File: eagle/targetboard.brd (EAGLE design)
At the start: 99.7 x 49.5 mm, 74 parts, among them CN1 DIP-BLACK-MALE-HEADER-VERT(3P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, IC1 TB6612FNG, IC2 TB6612FNG, IC3 MCP2551, IC4 MCP2551, IC5 LPC1768 or LPC1768, IC6 PMIC-CJT1117-3.3(SOT223), IC7 MAX232D, J1 USB, J2 Serial, J3 CAN, J4 2x8p-2.54, J5 2x8p-2.54, J6 DIP-BLACK-MALE-HEADER-VERT(8P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, J7 2x8p-2.54, Q1 PNP-24V, SW1 SW, Y1 12MHZ

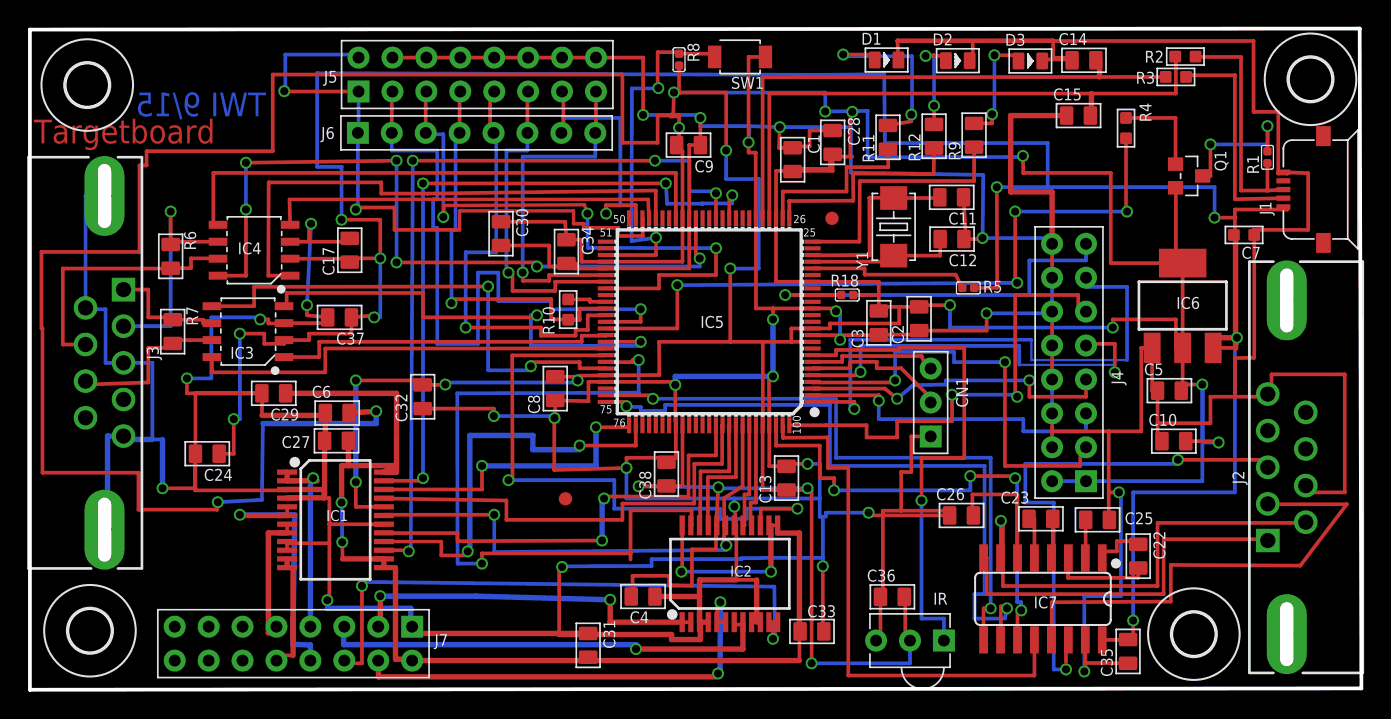
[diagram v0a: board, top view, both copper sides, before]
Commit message: Update of board
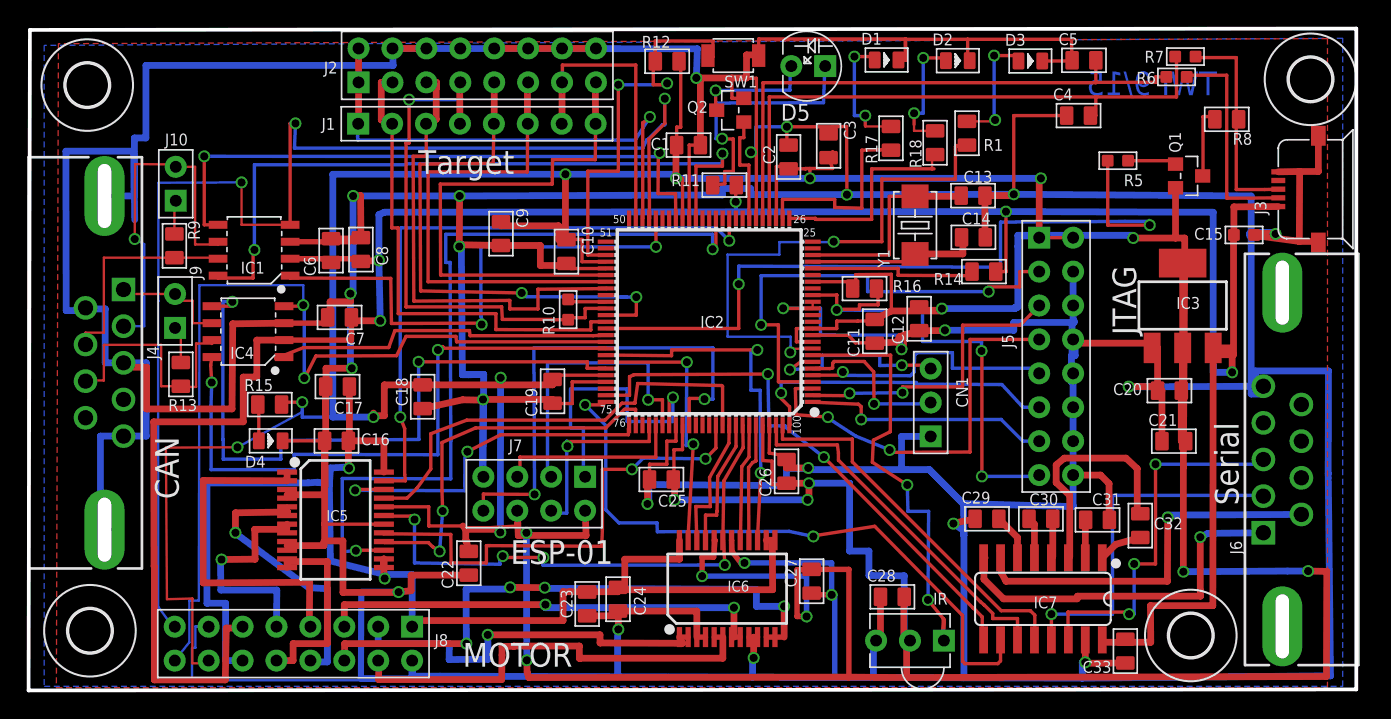
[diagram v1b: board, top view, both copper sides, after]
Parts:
- removed C34, C35, C37, C38: 100nf, Seeed-OPL-Capacitor:C0805
- removed C36: 10uf, Seeed-OPL-Capacitor:C0805
- removed R2, R3: 33.2R, Seeed-OPL-Resistor:R0603
- removed R4: 51R, Seeed-OPL-Resistor:R0603
- removed U$4, U$5: (no value), dicons:FIDUCIAL_G10
- added C16, C18, C21: 10uf, Seeed-OPL-Capacitor:C0805
- added C19, C20: 100nf, Seeed-OPL-Capacitor:C0805
- added D4: SMD-LED-CLEAR-RED(0805), Seeed-OPL-Diode:LED-0805
- added D5: IR 940NM, Seeed-OPL-Diode:LED2-2.54-D5.0MM
- added J10: CAN1, Seeed-OPL-Connector:H2-2.54
- added J8: 2x8p-2.54, Seeed-OPL-Connector:H2X8-2.54
- added J9: CAN2, Seeed-OPL-Connector:H2-2.54
- added Q2: NMOSFET, Seeed-OPL-Transistor:SOT-23
- added R13: 120R, Seeed-OPL-Resistor:R0805
- added R14: 1.5K, Seeed-OPL-Resistor:R0805
- added R15: 100R, Seeed-OPL-Resistor:R0805
- added R16: 2K, Seeed-OPL-Resistor:R0805
- added R17: 390R, Seeed-OPL-Resistor:R0805
- C10, C27: value 10uf -> 100nf
- C11, C12: value 18pf -> 100nf
- C13, C4, C5: value 100nf -> 18pf
- C15: value 18pf -> 10uf; device Seeed-OPL-Capacitor:C0805 -> Seeed-OPL-Capacitor:C0603
- C22, C23, C25, C26: value 1uf -> 100nf
- C24: value 1uf -> 10uf
- C29, C30, C6: value 100nf -> 1uf
- C3: value 100nf -> 10uf
- C31, C32: value 10uf -> 1uf
- C7: value 10uf -> 100nf; device Seeed-OPL-Capacitor:C0603 -> Seeed-OPL-Capacitor:C0805
- IC1: value TB6612FNG -> MCP2551; device Seeed-OPL-ic:SSOP24-0.65-8.9X5.3MM -> Seeed-OPL-ic:SOIC8-1.27-5X4MM
- IC2: value TB6612FNG -> LPC1768 or LPC1768; device Seeed-OPL-ic:SSOP24-0.65-8.9X5.3MM -> Seeed-OPL-ic:LQFP100-0.5-13.8X13.8MM
- IC3: value MCP2551 -> PMIC-CJT1117-3.3(SOT223); device Seeed-OPL-ic:SOIC8-1.27-5X4MM -> Seeed-OPL-ic:SOT-223
- IC5: value LPC1768 or LPC1768 -> TB6612FNG; device Seeed-OPL-ic:LQFP100-0.5-13.8X13.8MM -> Seeed-OPL-ic:SSOP24-0.65-8.9X5.3MM
- IC6: value PMIC-CJT1117-3.3(SOT223) -> TB6612FNG; device Seeed-OPL-ic:SOT-223 -> Seeed-OPL-ic:SSOP24-0.65-8.9X5.3MM
- J1: value USB -> DIP-BLACK-MALE-HEADER-VERT(8P-2.54); device Seeed-OPL-Connector:MICRO-USB5+2P-SMD-0.65 -> Seeed-OPL-Connector:H8-2.54
- J2: value Serial -> 2x8p-2.54; device Seeed-OPL-Connector:DSUB9+2P-2.77-90D-MALE -> Seeed-OPL-Connector:H2X8-2.54
- J3: value CAN -> USB; device Seeed-OPL-Connector:DSUB9+2P-2.77-90D-MALE -> Seeed-OPL-Connector:MICRO-USB5+2P-SMD-0.65
- J4: value 2x8p-2.54 -> CAN; device Seeed-OPL-Connector:H2X8-2.54 -> Seeed-OPL-Connector:DSUB9+2P-2.77-90D-MALE
- J6: value DIP-BLACK-MALE-HEADER-VERT(8P-2.54) -> Serial; device Seeed-OPL-Connector:H8-2.54 -> Seeed-OPL-Connector:DSUB9+2P-2.77-90D-MALE
- J7: value 2x8p-2.54 -> 2X4P-2.54; device Seeed-OPL-Connector:H2X8-2.54 -> Seeed-OPL-Connector:H2X4-2.54
- R1, R18: value 1.5K -> 390R; device Seeed-OPL-Resistor:R0402 -> Seeed-OPL-Resistor:R0805
- R11: value 2K -> 100R
- R12: value 2K -> 1.5K
- R5: value 1.5K -> 51R; device Seeed-OPL-Resistor:R0402 -> Seeed-OPL-Resistor:R0603
- R6, R7: value 120R -> 33.2R; device Seeed-OPL-Resistor:R0805 -> Seeed-OPL-Resistor:R0603
- R8: device Seeed-OPL-Resistor:R0402 -> Seeed-OPL-Resistor:R0805
- R9: value 2K -> 120R
- moved H3 100.3 mm to (4.78, 4.42)
- moved H4 92.4 mm to (87.2, 4.06)
- moved J3 88.9 mm to (93.8, 37.5), turned to 90 degrees
- moved R7 78.6 mm to (86.8, 47.4), turned to 90 degrees
- moved R6 76.5 mm to (86.2, 45.9), turned to 90 degrees
- moved J4 72.2 mm to (5.87, 24.5), turned to 270 degrees
- moved IC3 70.0 mm to (86.6, 28.8), turned to 0 degrees
- moved C7 68.0 mm to (23.5, 27.9)
- moved J2 67.7 mm to (33.8, 46.8)
- moved J6 65.1 mm to (94.1, 17.2)
- moved J1 60.6 mm to (33.8, 42.4)
- moved R9 60.5 mm to (11.1, 33.2), turned to 0 degrees
- moved C32 54.6 mm to (83.4, 12.3)
- moved C29 54.2 mm to (72.0, 12.8), turned to 90 degrees
- moved C22 50.1 mm to (33.1, 9.47), turned to 180 degrees
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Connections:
- removed net N$12: IC5.98, IC7.11
- removed net N$28: J7.11
- removed net N$29: J7.10
- removed net N$30: J7.9
- removed net N$31: J7.8
- removed net N$32: J7.7
- removed net N$33: J7.6
- new net ESP_0: IC2.81, J7.2
- new net ESP_2: IC2.80, J7.3
- new net ESP_RST: IC2.79, J7.7
- new net IR_SEND: IC2.32, Q2.1
- new net N$11: J10.1, R9.1
- new net N$14: D5.+, R11.1
- new net N$21: D5.-, Q2.3
- new net N$24: D4.+, R15.1
- new net RXD0: IC2.99, IC7.12
- new net RX_TO_TX: IC2.85, J7.5
- new net TXD0: IC2.98, IC7.11
- new net TX_TO_RX: IC2.82, J7.1
- net +12V: now also C16.2, C17.1, C23.1, C24.2, IC5.13, IC5.14, IC5.24, IC6.13, IC6.14, IC6.24, J8.1, J8.11; no longer C27.2, C29.1, C31.2, C33.1, IC1.13, IC1.14, IC1.24, IC2.13, IC2.14, IC2.24, J7.16
- net CAN1_H: now also IC1.7, J4.7, R9.2; no longer IC4.7, J3.7, R6.2
- net CAN1_L: now also IC1.6, J10.2, J4.2; no longer IC4.6, J3.2, R6.1
- net CAN1_REF: now also IC1.5, IC2.43; no longer IC4.5, IC5.43
- net CAN1_RS: now also IC1.8, IC2.40; no longer IC4.8, IC5.40
- net CAN1_RX: now also IC1.4, IC2.47, J8.8; no longer IC4.4, IC5.47
- net CAN1_TX: now also IC1.1, IC2.46; no longer IC4.1, IC5.46
- net CAN2_H: now also IC4.7, J4.8, R13.2; no longer IC3.7, J3.8, R7.2
- net CAN2_L: now also IC4.6, J4.1, J9.2; no longer IC3.6, J3.1, R7.1
- net CAN2_REF: now also IC2.70, IC4.5; no longer IC3.5, IC5.70
- net CAN2_RS: now also IC2.67, IC4.8; no longer IC3.8, IC5.67
- net CAN2_RX: now also IC2.66, IC4.4, J8.9; no longer IC3.4, IC5.66
- net CAN2_TX: now also IC2.65, IC4.1; no longer IC3.1, IC5.65
- net CM1A: now also IC2.91, IC6.22; no longer IC2.22, IC5.91
- net CM1B: now also IC2.92, IC6.21; no longer IC2.21, IC5.92
- net CM2A: now also IC2.94, IC6.17; no longer IC2.17, IC5.94
- net CM2B: now also IC2.95, IC6.16; no longer IC2.16, IC5.95
- net CM3A: now also IC2.76, IC5.22; no longer IC1.22, IC5.76
- net CM3B: now also IC2.90, IC5.21; no longer IC1.21, IC5.90
- net CM4A: now also IC2.89, IC5.17; no longer IC1.17, IC5.89
- net CM4B: now also IC2.77, IC5.16; no longer IC1.16, IC5.77
- net DM: now also J3.2, R6.2; no longer J1.2, R3.2
- net DP: now also J3.3, R7.2, R8.1; no longer J1.3, R1.1, R2.2
- net EDM: now also C5.2, IC2.30, R6.1; no longer C14.2, IC5.30, R3.1
- net EDP: now also C4.2, IC2.29, R7.1; no longer C15.2, IC5.29, R2.1
- net GND: now also C10.2, C13.1, C16.1, C18.1, C19.1, C20.1, C21.1, C22.1, C23.2, C24.1, C26.2, C29.1, C31.2, C33.1, C6.2, C7.2, C8.2, C9.2, D4.-, IC2.11, IC2.15, IC2.16, IC2.31, IC2.41, IC2.55, IC2.72, IC2.83, IC2.97, IC3.1, IC5.10, IC5.18, IC5.3, IC5.4, IC5.9, IC6.10, IC6.18, IC6.3, IC6.4, IC6.9, J2.10, J2.11, J2.12, J2.13, J2.14, J2.15, J2.9, J3.7, J4.3, J4.5, J4.6, J4.G1, J4.G2, J6.5, J7.4, J8.16, J8.7, Q2.2; no longer C10.1, C13.2, C24.2, C26.1, C29.2, C30.2, C31.1, C32.1, C33.2, C34.2, C35.1, C36.1, C37.2, C38.2, C6.1, C7.1, C8.1, C9.1, IC1.10, IC1.18, IC1.4, IC1.9, IC2.10, IC2.18, IC2.3, IC2.4, IC2.9, IC3.3, IC5.11, IC5.15, IC5.31, IC5.41, IC5.55, IC5.72, IC5.83, IC5.97, IC6.1, J1.5, J2.5, J2.7, J3.3, J3.G1, J3.G2, J4.10, J4.11, J4.12, J4.13, J4.14, J4.15, J4.9, J7.1
- net IR_IN: now also IC2.8; no longer IC5.8
- net LED1: now also IC2.9, R1.1; no longer IC5.25, R9.1
- net LED2: now also IC2.27, R17.1; no longer IC5.27, R11.1
- net LED3: now also IC2.26, R18.1; no longer IC5.26, R12.1
- net M1A: now also IC6.1, IC6.2, J8.2; no longer IC2.1, IC2.2, J7.2
- net M1B: now also IC6.5, IC6.6, J8.15; no longer IC2.5, IC2.6, J7.15
- net M2A: now also IC6.7, IC6.8, J8.3; no longer IC2.7, IC2.8, J7.3
- net M2B: now also IC6.11, IC6.12, J8.14; no longer IC2.11, IC2.12, J7.14
- net M3A: now also IC5.1, IC5.2, J8.4; no longer IC1.1, IC1.2, J7.4
- net M3B: now also IC5.5, IC5.6, J8.13; no longer IC1.5, IC1.6, J7.13
- net M4A: now also IC5.7, IC5.8, J8.5; no longer IC1.7, IC1.8, J7.5
- net M4B: now also IC5.11, IC5.12, J8.12; no longer IC1.11, IC1.12, J7.12
- net N$1: now also IC2.48, J1.1, J2.1, J2.16; no longer IC5.48, J5.1, J5.16, J6.1
- net N$10: now also IC2.21, R14.2; no longer IC5.21, R5.1
- net N$13: now also J9.1, R13.1; no longer IC5.99, IC7.12
- net N$15: now also C30.2; no longer C23.2
- net N$16: now also C30.1; no longer C23.1
- net N$17: now also C32.1; no longer C22.1
- net N$18: now also C32.2; no longer C22.2
- net N$19: now also C29.2; no longer C26.2
- net N$2: now also IC2.53, R12.1; no longer IC5.53, R8.1
- net N$20: now also C31.1; no longer C25.1
- net N$22: now also IC2.60; no longer IC5.60
- net N$3: now also R18.2; no longer R12.2
- net N$4: now also R17.2; no longer R11.2
- net N$5: now also R1.2; no longer R9.2
- net N$6: now also C14.2, IC2.22; no longer C12.2, IC5.22
- net N$7: now also R8.2; no longer R1.2
- net N$8: now also C13.2, IC2.23; no longer C11.2, IC5.23
- net N$9: now also R5.2; no longer R4.2
- net NTRST: now also IC2.4, J5.2; no longer IC5.4, J4.2
- net P2_9: now also IC2.64, R5.1; no longer IC5.64, R4.1
- net PWM1: now also IC2.69, IC6.23; no longer IC2.23, IC5.69
- net PWM2: now also IC2.68, IC6.15; no longer IC2.15, IC5.68
- net PWM3: now also IC2.35, IC5.23; no longer IC1.23, IC5.35
- net PWM4: now also IC2.37, IC5.15; no longer IC1.15, IC5.37
- net RST: now also IC2.17, J5.8, R16.1; no longer IC5.17, J4.8, R18.1
- net RTCK: now also IC2.100, J5.6; no longer IC5.100, J4.6
- net RX3: now also IC2.6; no longer IC5.6
- net RXD1: now also IC2.74; no longer IC5.74
- net SER1_RX: now also J6.2; no longer J2.2
- net SER1_TX: now also J6.3; no longer J2.3
- net SER2_RX: now also J6.1; no longer J2.1
- net SER2_TX: now also J6.6; no longer J2.6
- net STBY: now also IC2.93, IC5.19, IC6.19; no longer IC1.19, IC2.19, IC5.93
- net TCK: now also IC2.5, J5.5; no longer IC5.5, J4.5
- net TDI: now also IC2.2, J5.3; no longer IC5.2, J4.3
- net TDO: now also IC2.1, J5.7; no longer IC5.1, J4.7
- net TMS: now also IC2.3, J5.4; no longer IC5.3, J4.4
- net TX3: now also IC2.7; no longer IC5.7
- net TXD1: now also IC2.75; no longer IC5.75
- net T_RTCK: now also IC2.57, J1.6, J2.6; no longer IC5.57, J5.6, J6.6
- net T_SRST: now also IC2.56, J1.8, J2.8; no longer IC5.56, J5.8, J6.8
- net T_SWDCLK: now also IC2.62, J1.5, J2.5; no longer IC5.62, J5.5, J6.5
- net T_SWDIO: now also IC2.61, J1.4, J2.4; no longer IC5.61, J5.4, J6.4
- net T_SWO: now also IC2.49, J1.7, J2.7; no longer IC5.49, J5.7, J6.7
- net T_TDI: now also IC2.58, J1.3, J2.3; no longer IC5.58, J5.3, J6.3
- net T_TRST: now also IC2.63, J1.2, J2.2; no longer IC5.63, J5.2, J6.2
- net VCC: now also C15.2, C33.2, C6.1, C7.1, C8.1, IC1.2, IC3.3, J3.1, J8.6, R11.2, R14.1; no longer C17.1, C24.1, C35.2, C37.1, C7.2, IC3.2, IC6.3, J1.1, R5.2
- net VDD: now also C10.1, C11.2, C12.2, C18.2, C19.2, C20.2, C21.2, C22.2, C25.1, C26.1, C27.2, C9.1, IC2.10, IC2.12, IC2.19, IC2.28, IC2.42, IC2.54, IC2.71, IC2.84, IC2.96, IC3.2, IC3.TER, IC5.20, IC6.20, J5.1, J5.16, J7.6, J7.8, J8.10, R12.2, R15.2, R16.2; no longer C10.2, C13.1, C30.1, C32.2, C34.1, C36.2, C38.1, C4.2, C5.2, C6.2, C8.2, C9.2, IC1.20, IC2.20, IC5.10, IC5.12, IC5.19, IC5.28, IC5.42, IC5.54, IC5.71, IC5.84, IC5.96, IC6.2, IC6.TER, J4.1, J4.16, R18.2, R8.2
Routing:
- net GND: track 699.1 -> 835.9 mm, vias 27 -> 25
- net CAN1_RX: track 30.2 -> 97.0 mm, vias 0 -> 3
- net N$13: track 40.3 -> 3.02 mm
- net RX_TO_TX: track 0.00 -> 37.1 mm, vias 0 -> 2
- net N$12: track 36.9 -> 0.00 mm, vias 4 -> 0
- net PWM1: track 54.8 -> 20.1 mm
- net CAN2_RX: track 35.8 -> 70.5 mm
- net RXD0: track 0.00 -> 28.3 mm
- net TXD0: track 0.00 -> 27.3 mm
- net LED1: track 19.1 -> 41.6 mm, vias 0 -> 2
- net ESP_0: track 0.00 -> 22.1 mm, vias 0 -> 1
- net TX_TO_RX: track 0.00 -> 22.0 mm, vias 0 -> 1
- net TDO: track 40.6 -> 18.7 mm
- net N$14: track 0.00 -> 19.7 mm, vias 0 -> 1
- net PWM2: track 46.0 -> 27.3 mm
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- added copper zone on layer 1, net GND
- added copper zone on layer 16, net GND
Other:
- board size 99.7 x 49.5 mm -> 99.4 x 49.6 mm
- board text added: "CAN"
- board text added: "ESP-01"
- board text added: "JTAG"
- board text added: "MOTOR"
- board text added: "Serial"
- board text added: "Target"
- board text removed: "Targetboard"
